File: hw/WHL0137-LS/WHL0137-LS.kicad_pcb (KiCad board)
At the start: 4 copper layers, 111.5 x 124.3 mm, 91 parts, among them J1 Conn_01x05, U1 IS31FL3236A, U2 IS31FL3236A

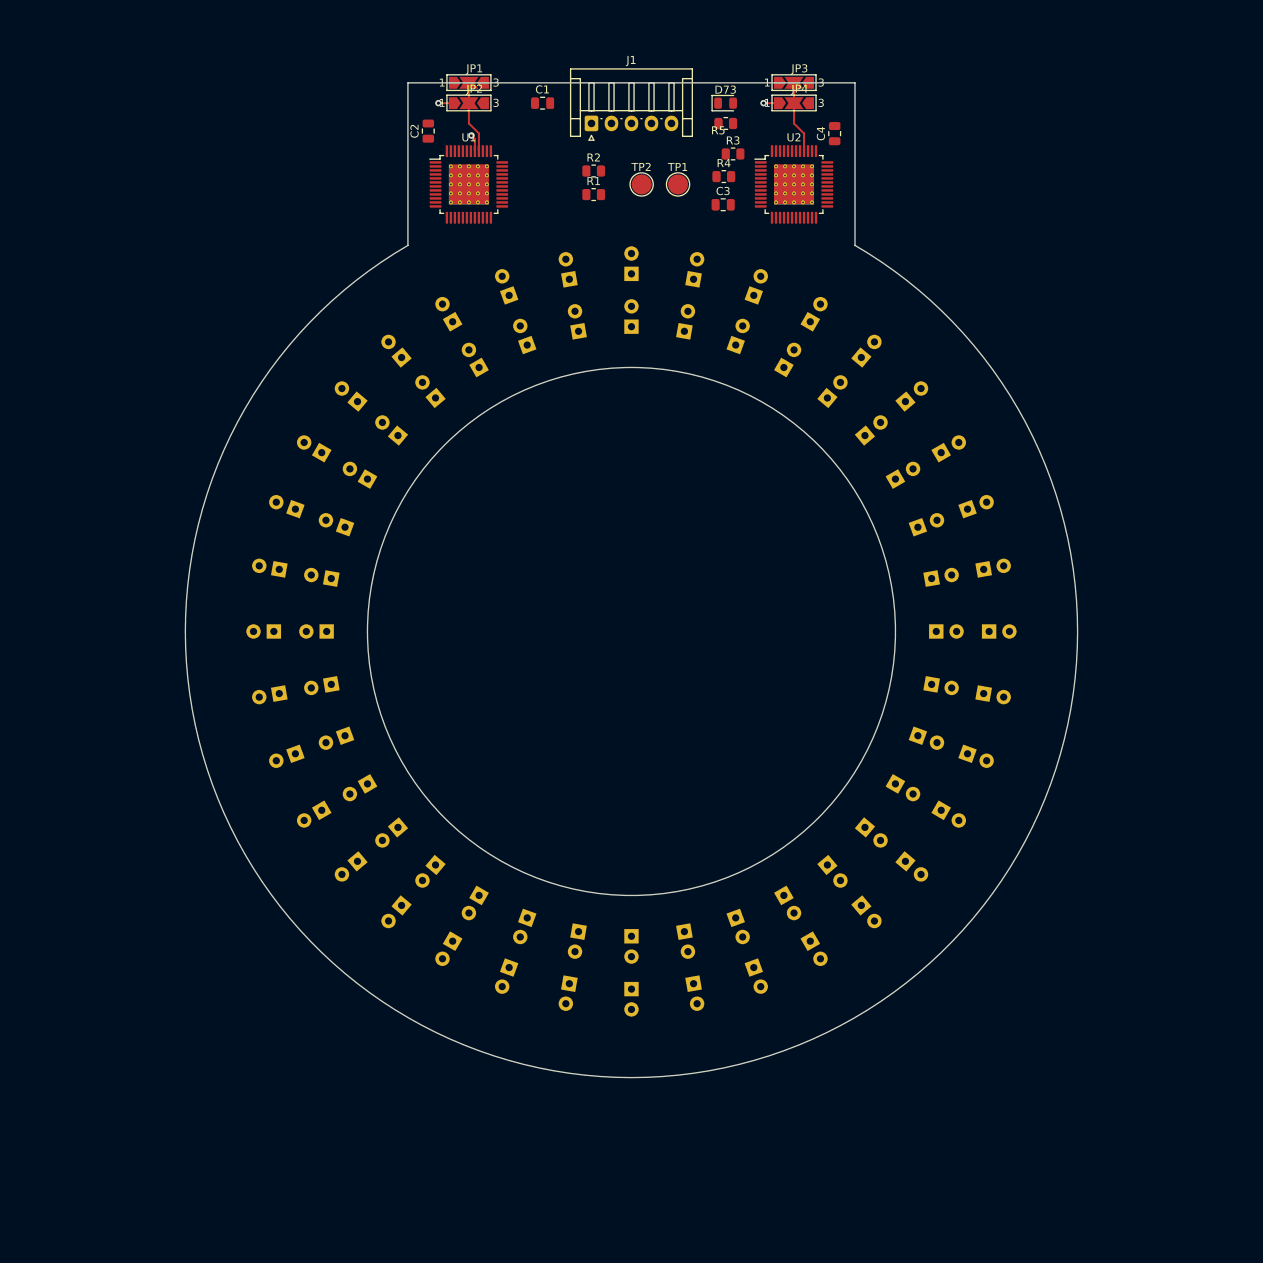
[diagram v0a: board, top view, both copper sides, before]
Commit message: Some layout
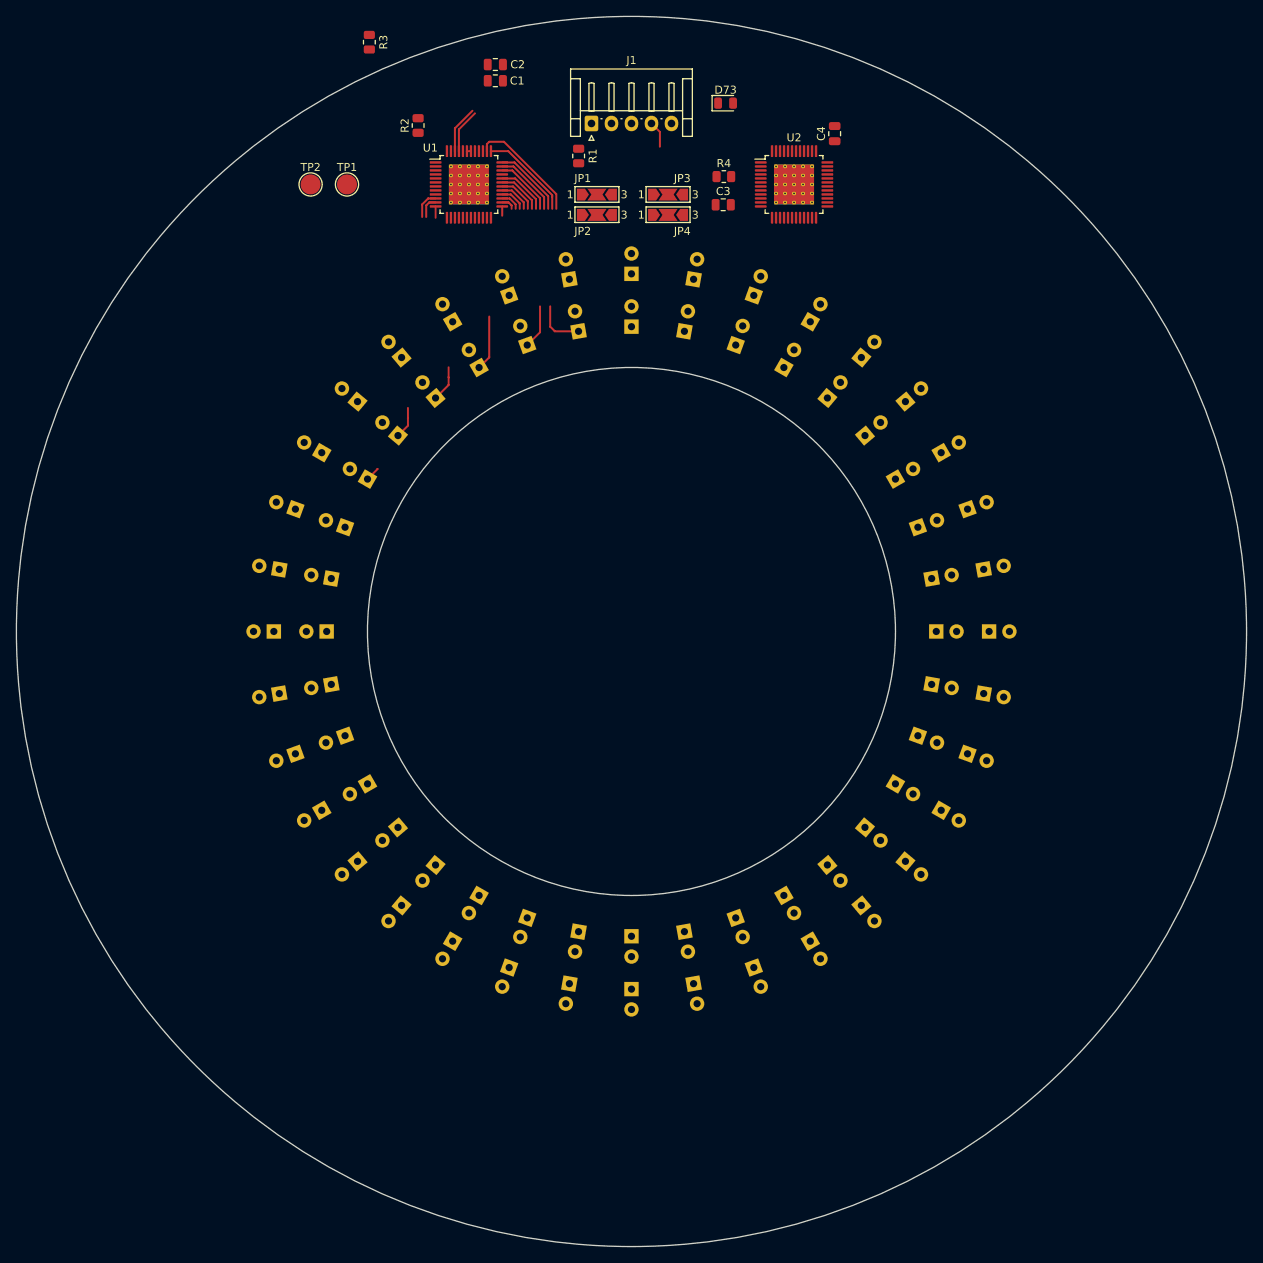
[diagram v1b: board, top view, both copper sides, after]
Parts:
- removed R5: 510, Resistor_SMD:R_0805_2012Metric
- R1: value 100k -> 510
- R2: value 3.3k -> 100k
- R3: value 100k -> 3.3k
- moved R3 47.6 mm to (-32.8, -73.7), turned to 90 degrees
- moved TP1 41.4 mm to (-35.6, -55.9)
- moved TP2 41.4 mm to (-40.1, -55.9)
- moved R2 22.7 mm to (-26.7, -63.2), turned to 90 degrees
- moved JP2 21.2 mm to (-4.32, -52.1)
- moved JP1 21.2 mm to (-4.32, -54.6)
- moved JP4 21.1 mm to (4.57, -52.1)
- moved JP3 21.1 mm to (4.57, -54.6)
- moved C2 11.8 mm to (-17.0, -70.9), turned to 0 degrees
- moved C1 6.54 mm to (-17.0, -68.8)
- moved R1 5.18 mm to (-6.60, -59.4), turned to 90 degrees
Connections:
- D1 pad 1: Net-(U1-Pad47) -> Net-(D1-Pad1)
- D2 pad 1: Net-(U1-Pad48) -> Net-(D2-Pad1)
- D28 pad 1: Net-(U1-Pad38) -> Net-(D28-Pad1)
- D29 pad 1: Net-(U1-Pad37) -> Net-(D29-Pad1)
- D3 pad 1: Net-(U1-Pad1) -> Net-(D3-Pad1)
- D37 pad 1: Net-(U2-Pad8) -> Net-(D37-Pad1)
- D38 pad 1: Net-(U2-Pad7) -> Net-(D38-Pad1)
- D39 pad 1: Net-(U2-Pad6) -> Net-(D39-Pad1)
- D4 pad 1: Net-(U1-Pad2) -> Net-(D4-Pad1)
- D40 pad 1: Net-(U2-Pad5) -> Net-(D40-Pad1)
- D41 pad 1: Net-(U2-Pad3) -> Net-(D41-Pad1)
- D42 pad 1: Net-(U2-Pad2) -> Net-(D42-Pad1)
- D43 pad 1: Net-(U2-Pad1) -> Net-(D43-Pad1)
- D44 pad 1: Net-(U2-Pad48) -> Net-(D44-Pad1)
- D45 pad 1: Net-(U2-Pad47) -> Net-(D45-Pad1)
- D5 pad 1: Net-(U1-Pad3) -> Net-(D5-Pad1)
- D6 pad 1: Net-(U1-Pad5) -> Net-(D6-Pad1)
- D7 pad 1: Net-(U1-Pad6) -> Net-(D7-Pad1)
- D8 pad 1: Net-(U1-Pad7) -> Net-(D8-Pad1)
- D9 pad 1: Net-(U1-Pad8) -> Net-(D9-Pad1)
- R1 pad 1: GND -> +5V
- R1 pad 2: /inner_LED_ring/SDB -> Net-(D73-Pad2)
- R2 pad 1: Net-(U1-Pad44) -> /inner_LED_ring/SDB
- R3 pad 1: GND -> Net-(R3-Pad1)
- R3 pad 2: /inner_LED_ring/SDB -> GND
- U1 pad 1: Net-(U1-Pad1) -> Net-(D14-Pad1)
- U1 pad 10: Net-(D11-Pad1) -> Net-(D5-Pad1)
- U1 pad 11: Net-(D12-Pad1) -> Net-(D7-Pad1)
- U1 pad 12: Net-(D13-Pad1) -> Net-(D9-Pad1)
- U1 pad 13: Net-(D14-Pad1) -> Net-(D11-Pad1)
- U1 pad 14: Net-(D15-Pad1) -> Net-(D13-Pad1)
- U1 pad 15: Net-(D16-Pad1) -> Net-(D15-Pad1)
- U1 pad 17: Net-(D18-Pad1) -> Net-(D19-Pad1)
- U1 pad 2: Net-(U1-Pad2) -> Net-(D12-Pad1)
- U1 pad 20: Net-(D19-Pad1) -> Net-(D20-Pad1)
- U1 pad 21: Net-(D20-Pad1) -> Net-(D22-Pad1)
- U1 pad 22: Net-(D21-Pad1) -> Net-(D24-Pad1)
- U1 pad 23: Net-(D22-Pad1) -> Net-(D26-Pad1)
- U1 pad 24: Net-(D23-Pad1) -> Net-(D28-Pad1)
- U1 pad 25: Net-(D24-Pad1) -> Net-(D30-Pad1)
- U1 pad 26: Net-(D25-Pad1) -> Net-(D32-Pad1)
- U1 pad 27: Net-(D26-Pad1) -> Net-(D34-Pad1)
- U1 pad 28: Net-(D27-Pad1) -> Net-(D36-Pad1)
- U1 pad 29: Net-(D36-Pad1) -> Net-(D37-Pad1)
- U1 pad 3: Net-(U1-Pad3) -> Net-(D10-Pad1)
- U1 pad 31: Net-(D34-Pad1) -> Net-(D33-Pad1)
- U1 pad 32: Net-(D33-Pad1) -> Net-(D31-Pad1)
- U1 pad 34: Net-(D32-Pad1) -> Net-(D29-Pad1)
- U1 pad 35: Net-(D31-Pad1) -> Net-(D27-Pad1)
- U1 pad 36: Net-(D30-Pad1) -> Net-(D25-Pad1)
- U1 pad 37: Net-(U1-Pad37) -> Net-(D23-Pad1)
- U1 pad 38: Net-(U1-Pad38) -> Net-(D21-Pad1)
- U1 pad 44: Net-(U1-Pad44) -> Net-(R3-Pad1)
- U1 pad 47: Net-(U1-Pad47) -> Net-(D18-Pad1)
- U1 pad 48: Net-(U1-Pad48) -> Net-(D16-Pad1)
- U1 pad 5: Net-(U1-Pad5) -> Net-(D8-Pad1)
- U1 pad 6: Net-(U1-Pad6) -> Net-(D6-Pad1)
- U1 pad 7: Net-(U1-Pad7) -> Net-(D4-Pad1)
- U1 pad 8: Net-(U1-Pad8) -> Net-(D2-Pad1)
- U1 pad 9: Net-(D10-Pad1) -> Net-(D3-Pad1)
- U2 pad 1: Net-(U2-Pad1) -> Net-(D50-Pad1)
- U2 pad 10: Net-(D47-Pad1) -> Net-(D41-Pad1)
- U2 pad 11: Net-(D48-Pad1) -> Net-(D43-Pad1)
- U2 pad 12: Net-(D49-Pad1) -> Net-(D45-Pad1)
- U2 pad 13: Net-(D50-Pad1) -> Net-(D47-Pad1)
- U2 pad 14: Net-(D51-Pad1) -> Net-(D49-Pad1)
- U2 pad 15: Net-(D52-Pad1) -> Net-(D51-Pad1)
- U2 pad 17: Net-(D54-Pad1) -> Net-(D55-Pad1)
- U2 pad 2: Net-(U2-Pad2) -> Net-(D48-Pad1)
- U2 pad 20: Net-(D55-Pad1) -> Net-(D56-Pad1)
- U2 pad 21: Net-(D56-Pad1) -> Net-(D58-Pad1)
- U2 pad 22: Net-(D57-Pad1) -> Net-(D60-Pad1)
- U2 pad 23: Net-(D58-Pad1) -> Net-(D62-Pad1)
- U2 pad 24: Net-(D59-Pad1) -> Net-(D64-Pad1)
- U2 pad 25: Net-(D60-Pad1) -> Net-(D66-Pad1)
- U2 pad 26: Net-(D61-Pad1) -> Net-(D68-Pad1)
- U2 pad 27: Net-(D62-Pad1) -> Net-(D70-Pad1)
- U2 pad 28: Net-(D63-Pad1) -> Net-(D72-Pad1)
- U2 pad 29: Net-(D64-Pad1) -> Net-(D1-Pad1)
- U2 pad 3: Net-(U2-Pad3) -> Net-(D46-Pad1)
- U2 pad 30: Net-(D65-Pad1) -> Net-(D71-Pad1)
- U2 pad 31: Net-(D66-Pad1) -> Net-(D69-Pad1)
- U2 pad 34: Net-(D68-Pad1) -> Net-(D65-Pad1)
- U2 pad 35: Net-(D69-Pad1) -> Net-(D63-Pad1)
- U2 pad 36: Net-(D70-Pad1) -> Net-(D61-Pad1)
- U2 pad 37: Net-(D71-Pad1) -> Net-(D59-Pad1)
- U2 pad 38: Net-(D72-Pad1) -> Net-(D57-Pad1)
- U2 pad 47: Net-(U2-Pad47) -> Net-(D54-Pad1)
- U2 pad 48: Net-(U2-Pad48) -> Net-(D52-Pad1)
- U2 pad 5: Net-(U2-Pad5) -> Net-(D44-Pad1)
- U2 pad 6: Net-(U2-Pad6) -> Net-(D42-Pad1)
- U2 pad 7: Net-(U2-Pad7) -> Net-(D40-Pad1)
- U2 pad 8: Net-(U2-Pad8) -> Net-(D38-Pad1)
- U2 pad 9: Net-(D46-Pad1) -> Net-(D39-Pad1)
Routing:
- net Net-(D21-Pad1): track 0.00 -> 14.2 mm
- net Net-(D23-Pad1): track 0.00 -> 11.7 mm
- net Net-(D25-Pad1): track 0.00 -> 9.07 mm
- net Net-(JP3-Pad2): track 9.06 -> 0.00 mm
- net Net-(JP1-Pad2): track 9.06 -> 0.00 mm
- net Net-(D27-Pad1): track 0.00 -> 8.28 mm
- net Net-(D5-Pad1): track 0.00 -> 8.07 mm
- net Net-(D29-Pad1): track 0.00 -> 7.49 mm
- net Net-(D4-Pad1): track 0.00 -> 6.90 mm
- net Net-(D31-Pad1): track 0.00 -> 6.50 mm
- net Net-(D2-Pad1): track 0.00 -> 6.32 mm
- net /inner_LED_ring/SCL: track 0.00 -> 5.95 mm
- net +5V: track 5.78 -> 0.00 mm, vias 3 -> 0
- net Net-(D33-Pad1): track 0.00 -> 5.71 mm
- net /inner_LED_ring/SDA: track 0.00 -> 5.56 mm
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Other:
- board size 111.5 x 124.3 mm -> 153.8 x 153.8 mm
